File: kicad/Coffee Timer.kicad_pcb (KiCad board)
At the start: 2 copper layers, 78.7 x 53.3 mm, 28 parts, among them J1 Screw_Terminal_01x02, Q1 PN2222A, SW1 SW_Push, SW2 SW_Push, U1 ATtiny85-20PU, U3 74HC595, U4 74HC595

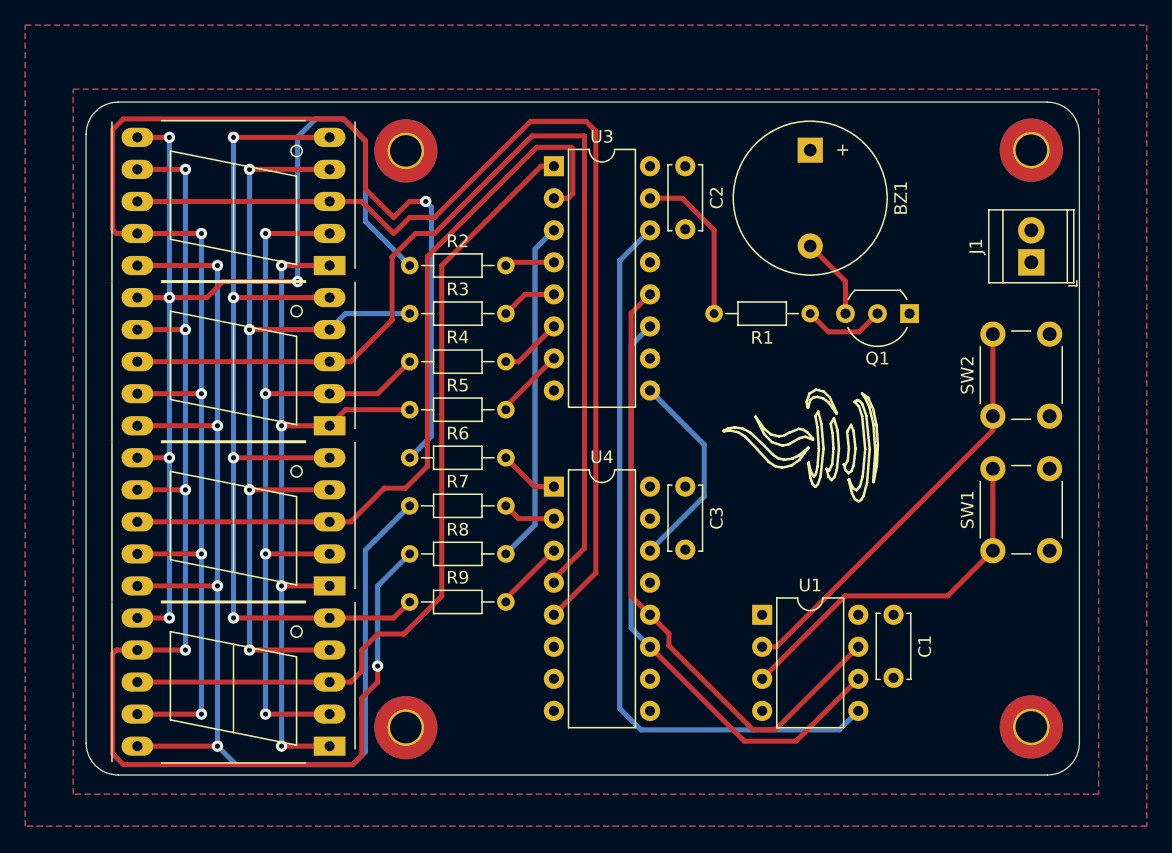
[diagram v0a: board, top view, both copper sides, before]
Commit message: fix
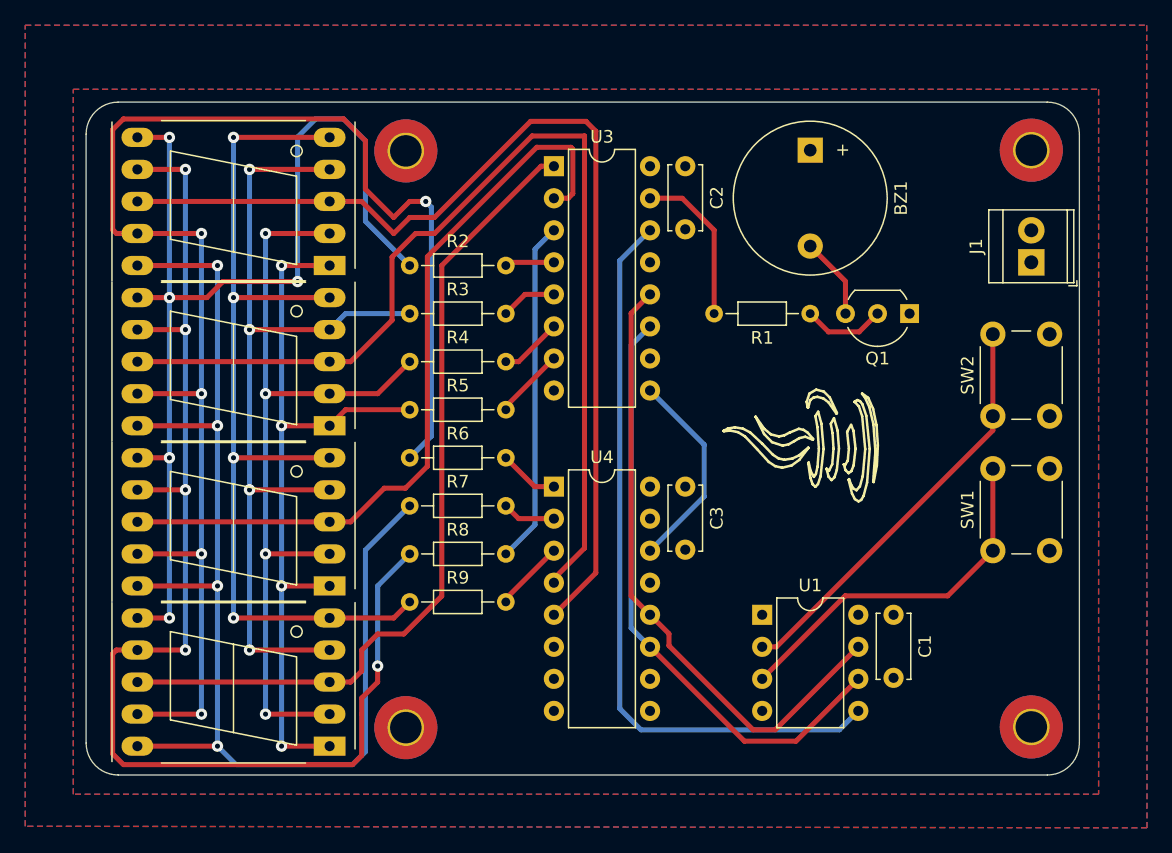
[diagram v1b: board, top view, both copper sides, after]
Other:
- net class Default: clearance 0.5 -> 0.3; trace_width 0.127 -> 0.4
- rule trace_clearance: 0.5 -> 0.3
- rule trace_min: 0.5 -> 0.4
